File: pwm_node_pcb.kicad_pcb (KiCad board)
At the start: 4 copper layers, 40 x 35 mm, 45 parts, among them J1 CAN1, J2 TC2050-IDC-NL, J3 Battery, J5 Load Source, J6 5V Breakout, U1 LMR51430, U2 TJA1051T/3, U3 LD1117S33CTR, U4 STM32L432KCU, U5 TXB0104QPWRQ1, Y1 ECS-2520MV-080-BN

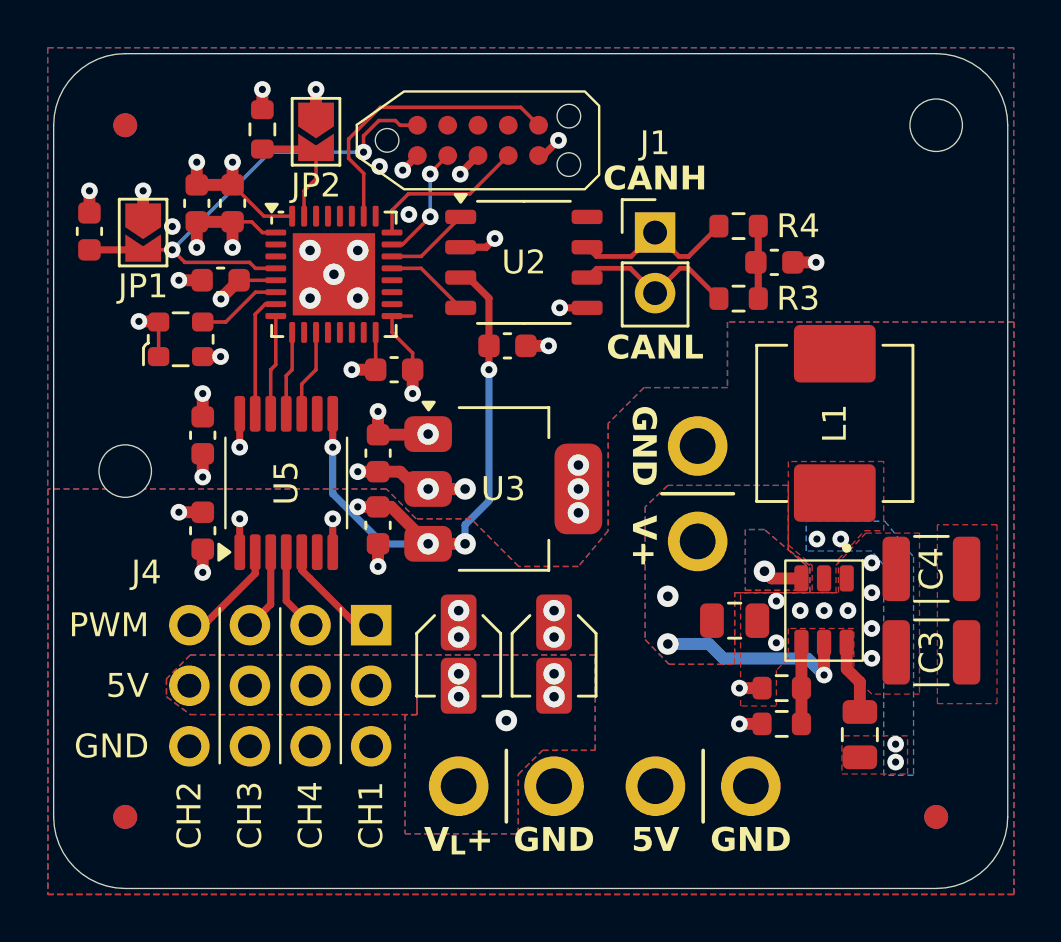
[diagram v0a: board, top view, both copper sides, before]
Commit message: Trace cleanup
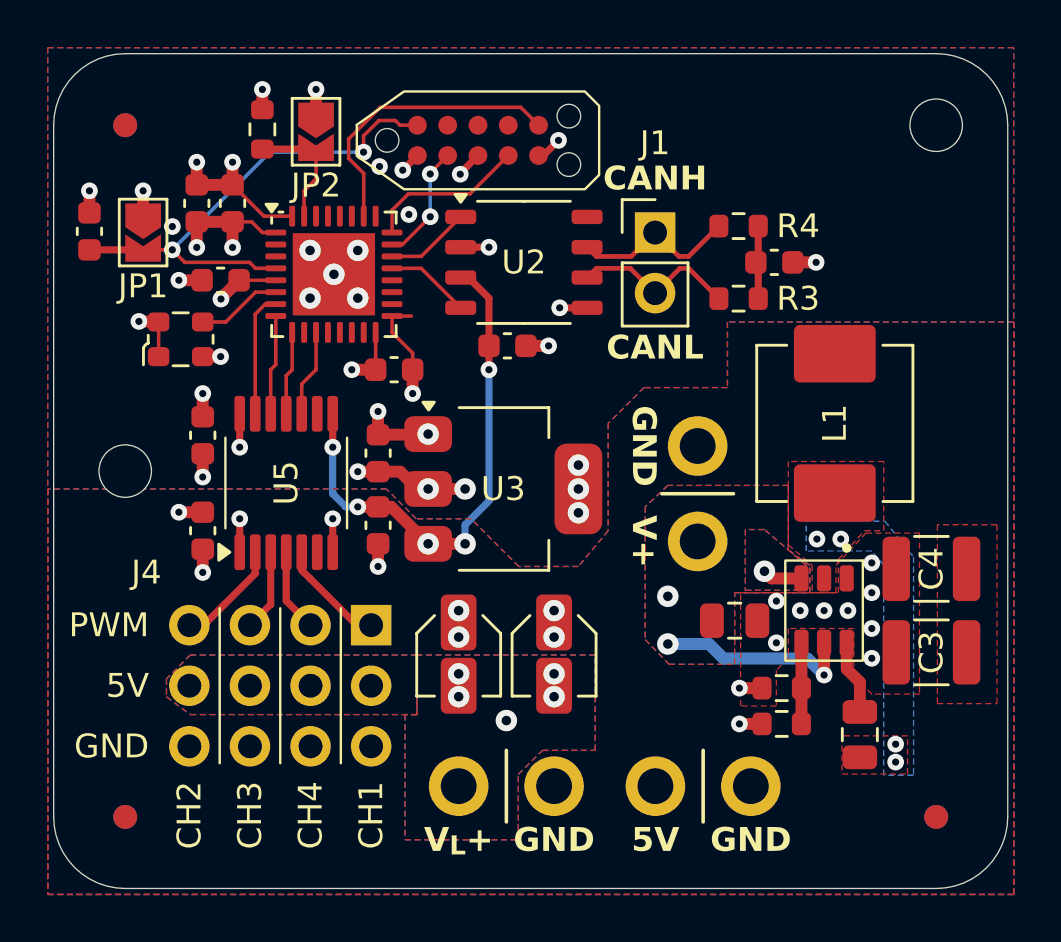
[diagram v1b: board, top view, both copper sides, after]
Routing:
- net +5V: track 29.4 -> 25.8 mm
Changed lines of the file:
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@@
-	)
-	(segment
-		(start 154.885 103.865)
-		(end 153.815 103.865)
-		(width 0.3)
-		(layer "F.Cu")
-		(net 1)
 	)
 	(segment
@@
 	)
 	(segment
-		(start 155.25 103.5)
-		(end 154.885 103.865)
-		(width 0.3)
-		(layer "F.Cu")
-		(net 1)
-	)
-	(segment
 		(start 144.25 101.25)
 		(end 144.25 100.3)
@@
 	)
 	(segment
+		(start 155 103.865)
+		(end 153.815 103.865)
+		(width 0.3)
+		(layer "F.Cu")
+		(net 1)
+	)
+	(segment
 		(start 143.75 108.45)
 		(end 143 108.45)
@@
 	)
 	(via
-		(at 155.25 103.5)
+		(at 155 103.865)
 		(size 0.7)
 		(drill 0.3)
@@
 	)
 	(segment
+		(start 149.5 114.75)
+		(end 149 114.75)
+		(width 0.3)
+		(layer "B.Cu")
+		(net 2)
+	)
+	(segment
 		(start 154 115.5)
 		(end 154 116.3)
@@
 	)
 	(segment
-		(start 150.55 116.3)
-		(end 148.45 114.2)
-		(width 0.3)
-		(layer "B.Cu")
-		(net 2)
-	)
-	(segment
-		(start 152.45 116.3)
-		(end 150.55 116.3)
-		(width 0.3)
-		(layer "B.Cu")
-		(net 2)
-	)
-	(segment
 		(start 148.45 114.2)
 		(end 148.45 112.25)
+		(width 0.3)
+		(layer "B.Cu")
+		(net 2)
+	)
+	(segment
+		(start 149 114.75)
+		(end 148.45 114.2)
 		(width 0.3)
 		(layer "B.Cu")
@@
 		(polygon
 			(pts
-				(xy 152.5 104.25) (xy 152.5 104.75) (xy 153 104.75) (xy 152.965 104.25)
+				(xy 152.5 104.25) (xy 152.5 104.75) (xy 153 104.75) (xy 153 104.25)
 			)
 		)
@@
 		(polygon
 			(pts
-				(xy 151.98 123.46) (xy 151.48 123.46) (xy 151.48 128.46) (xy 156.23 128.46) (xy 156.23 125.964951)
+				(xy 151.98 123.46) (xy 151.48 123.46) (xy 151.48 128.71) (xy 156.23 128.71) (xy 156.23 125.964951)
 				(xy 157.245 124.96) (xy 159.455 124.96) (xy 159.455 120.96) (xy 151.98 120.96)
 			)
